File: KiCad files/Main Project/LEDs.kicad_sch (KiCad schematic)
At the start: 11 parts, among them U10 WS2812-4020_dual, U11 WS2812-4020_dual, U12 WS2812-4020_dual, U13 WS2812-4020_dual, U14 WS2812-4020_dual, U15 WS2812-4020_dual, U5 WS2812-4020_dual, U6 WS2812-4020_dual, U7 WS2812-4020_dual, U8 WS2812-4020_dual, U9 WS2812-4020_dual

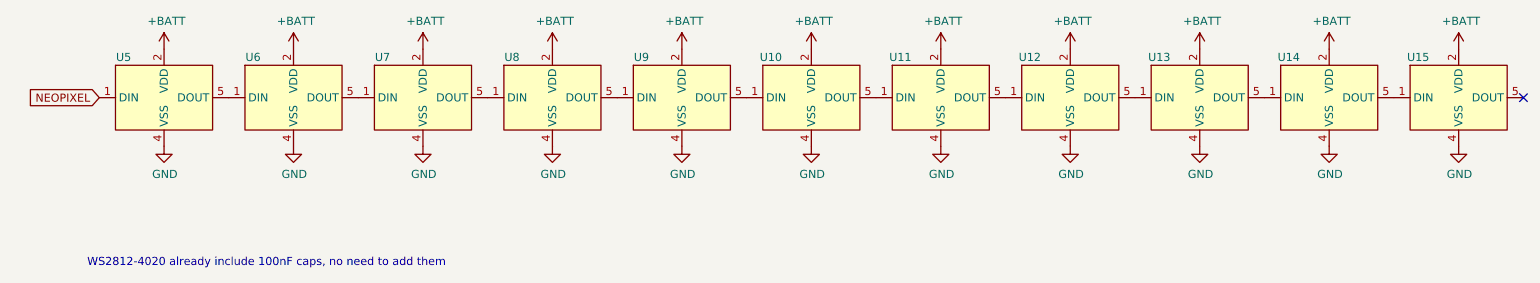
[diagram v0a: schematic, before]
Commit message: update
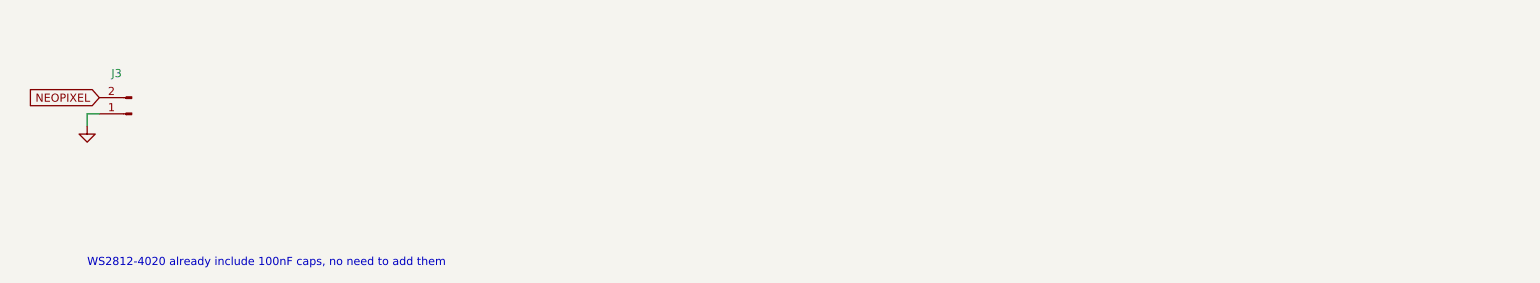
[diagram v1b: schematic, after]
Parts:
- removed U10, U11, U12, U13, U14, U15, U5, U6, U7, U8, U9: WS2812-4020_dual, Josip_global:WS2812-4020-dual-6mm_bezMaske, symbol Josip_symbol_global:WS2812-4020_dual
- added J3: (no value), symbol Connector:Conn_01x02_Male
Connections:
- net GND: now also J3.1 (Pin_1)
- net NEOPIXEL: now also J3.2 (Pin_2)
- no-connect marks 1 -> 0

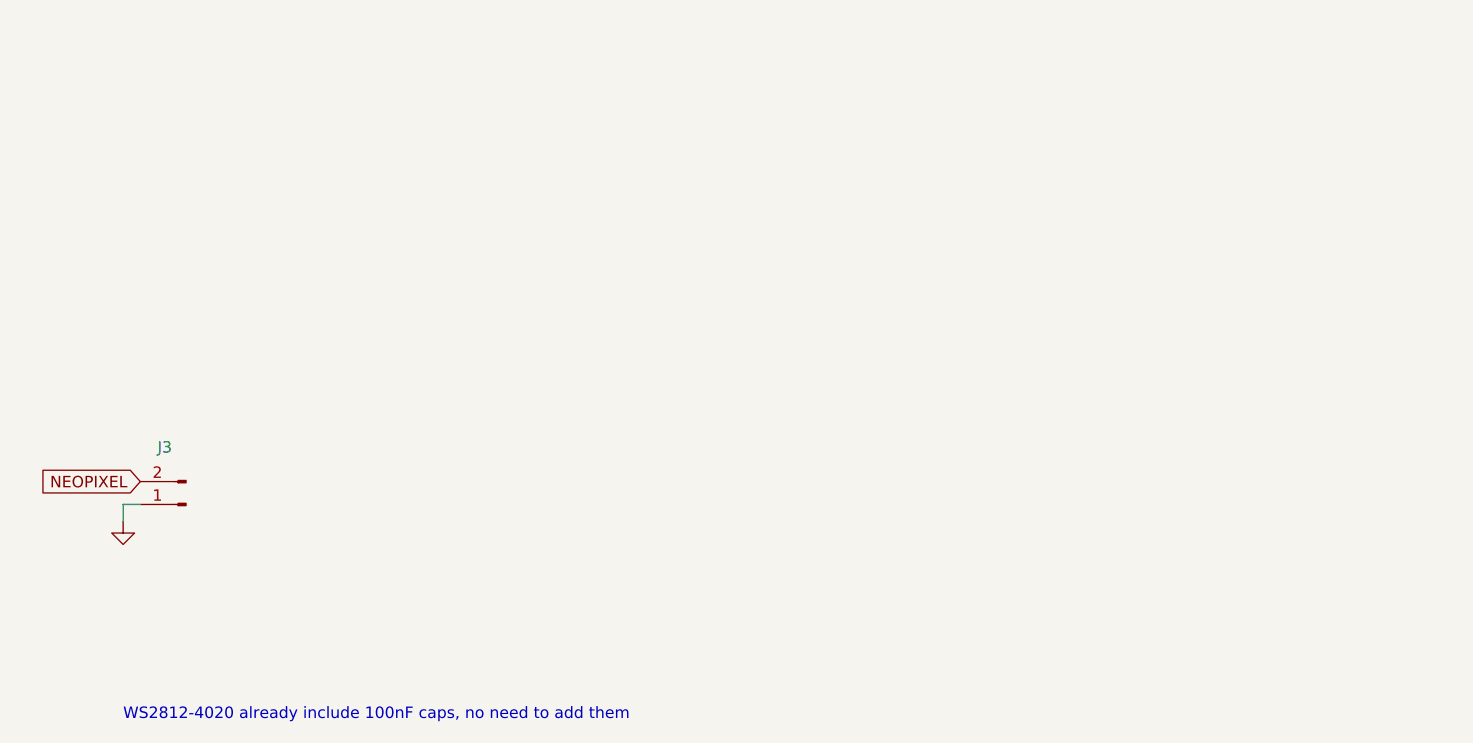
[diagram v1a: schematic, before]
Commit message: update
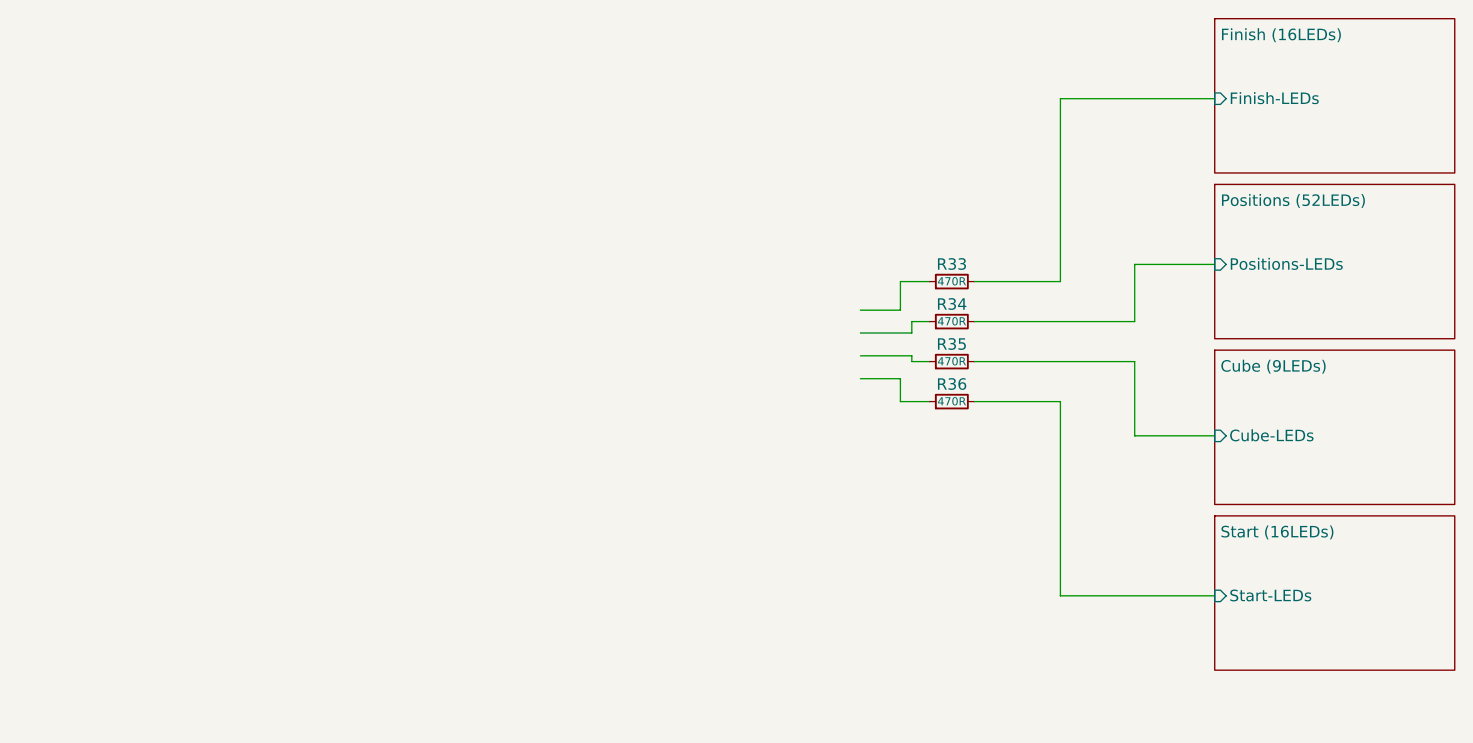
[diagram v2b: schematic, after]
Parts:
- removed J3: (no value), symbol Connector:Conn_01x02_Male
- added R33, R34, R35, R36: 470R, Resistor_SMD:R_0603_1608Metric, symbol Device:R_Small
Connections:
- new net Cube (9LEDs)/Cube-LEDs: R35.2
- new net Finish (16LEDs)/Finish-LEDs: R33.2
- new net Positions (52LEDs)/Positions-LEDs: R34.2
- new net Start (16LEDs)/Start-LEDs: R36.2
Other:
- added sheet Cube (9LEDs) (Cube.kicad_sch)
- added sheet Finish (16LEDs) (Finish.kicad_sch)
- added sheet Positions (52LEDs) (Positions.kicad_sch)
- added sheet Start (16LEDs) (Start.kicad_sch)
- note removed: "WS2812-4020 already include 100nF caps, no need to add them"
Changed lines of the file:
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@@
     (company "Josip&Zvonimir")
   )
-  (wire (pts (xy 42.545 100.965) (xy 42.545 99.06))
+  (wire (pts (xy 146.685 87.63) (xy 137.16 87.63))
     (stroke (width 0) (type default) (color 0 0 0 0))
   )
-  (wire (pts (xy 42.545 99.06) (xy 44.45 99.06))
+  (wire (pts (xy 130.175 80.01) (xy 130.175 78.74))
     (stroke (width 0) (type default) (color 0 0 0 0))
   )
-  (text "WS2812-4020 already include 100nF caps, no need to add them"
-    (at 42.545 123.19 0)
-    (effects (font (size 1.27 1.27)) (justify left bottom))
+  (wire (pts (xy 132.08 87.63) (xy 128.905 87.63))
+    (stroke (width 0) (type default) (color 0 0 0 0))
   )
-  (global_label "NEOPIXEL" (shape input) (at 44.45 96.52 180) (fields_autoplaced)
-    (effects (font (size 1.27 1.27)) (justify right))
-    (property "Intersheet References" "${INTERSHEET_REFS}" (id 0) (at -2.54 50.165 0)
+  (wire (pts (xy 128.905 87.63) (xy 128.905 85.09))
+    (stroke (width 0) (type default) (color 0 0 0 0))
+  )
+  (wire (pts (xy 163.83 72.39) (xy 154.94 72.39))
+    (stroke (width 0) (type default) (color 0 0 0 0))
+  )
+  (wire (pts (xy 137.16 74.295) (xy 146.685 74.295))
+    (stroke (width 0) (type default) (color 0 0 0 0))
+  )
+  (wire (pts (xy 146.685 53.975) (xy 163.83 53.975))
+    (stroke (width 0) (type default) (color 0 0 0 0))
+  )
+  (wire (pts (xy 137.16 83.185) (xy 154.94 83.185))
+    (stroke (width 0) (type default) (color 0 0 0 0))
+  )
+  (wire (pts (xy 124.46 77.47) (xy 128.905 77.47))
+    (stroke (width 0) (type default) (color 0 0 0 0))
+  )
+  (wire (pts (xy 146.685 74.295) (xy 146.685 53.975))
+    (stroke (width 0) (type default) (color 0 0 0 0))
+  )
+  (wire (pts (xy 146.685 109.22) (xy 146.685 87.63))
+    (stroke (width 0) (type default) (color 0 0 0 0))
+  )
+  (wire (pts (xy 128.905 77.47) (xy 128.905 74.295))
+    (stroke (width 0) (type default) (color 0 0 0 0))
+  )
+  (wire (pts (xy 163.83 109.22) (xy 146.685 109.22))
+    (stroke (width 0) (type default) (color 0 0 0 0))
+  )
+  (wire (pts (xy 124.46 82.55) (xy 130.175 82.55))
+    (stroke (width 0) (type default) (color 0 0 0 0))
+  )
+  (wire (pts (xy 124.46 80.01) (xy 130.175 80.01))
+    (stroke (width 0) (type default) (color 0 0 0 0))
+  )
+  (wire (pts (xy 128.905 74.295) (xy 132.08 74.295))
+    (stroke (width 0) (type default) (color 0 0 0 0))
+  )
+  (wire (pts (xy 154.94 83.185) (xy 154.94 91.44))
+    (stroke (width 0) (type default) (color 0 0 0 0))
+  )
+  (wire (pts (xy 154.94 78.74) (xy 137.16 78.74))
+    (stroke (width 0) (type default) (color 0 0 0 0))
+  )
+  (wire (pts (xy 154.94 72.39) (xy 154.94 78.74))
+    (stroke (width 0) (type default) (color 0 0 0 0))
+  )
+  (wire (pts (xy 130.175 78.74) (xy 132.08 78.74))
+    (stroke (width 0) (type default) (color 0 0 0 0))
+  )
+  (wire (pts (xy 154.94 91.44) (xy 163.83 91.44))
+    (stroke (width 0) (type default) (color 0 0 0 0))
+  )
+  (wire (pts (xy 130.175 82.55) (xy 130.175 83.185))
+    (stroke (width 0) (type default) (color 0 0 0 0))
+  )
+  (wire (pts (xy 130.175 83.185) (xy 132.08 83.185))
+    (stroke (width 0) (type default) (color 0 0 0 0))
+  )
+  (wire (pts (xy 128.905 85.09) (xy 124.46 85.09))
+    (stroke (width 0) (type default) (color 0 0 0 0))
+  )
+  (symbol (lib_id "Device:R_Small") (at 134.62 78.74 90) (unit 1)
+    (in_bom yes) (on_board yes)
+    (property "Reference" "R34" (id 0) (at 134.62 76.835 90))
+    (property "Value" "470R" (id 1) (at 134.62 78.74 90)
+      (effects (font (size 0.9 0.9)))
+    )
+    (property "Footprint" "Resistor_SMD:R_0603_1608Metric" (id 2) (at 134.62 78.74 0)
       (effects (font (size 1.27 1.27)) hide)
     )
-  )
-  (symbol (lib_id "Connector:Conn_01x02_Male") (at 49.53 99.06 180) (unit 1)
-    (in_bom yes) (on_board yes)
-    (property "Reference" "J3" (id 0) (at 46.355 92.71 0)
-      (effects (font (size 1.27 1.27)) (justify right))
-    )
-    (property "Value" "" (id 1) (at 50.2412 99.4922 0)
-      (effects (font (size 1.27 1.27)) (justify right) hide)
-    )
-    (property "Footprint" "" (id 2) (at 49.53 99.06 0)
-      (effects (font (size 1.27 1.27)) hide)
-    )
-    (property "Datasheet" "~" (id 3) (at 49.53 99.06 0)
+    (property "Datasheet" "~" (id 3) (at 134.62 78.74 0)
       (effects (font (size 1.27 1.27)) hide)
     )
@@
     (pin "2")
   )
-  (symbol (lib_id "power:GND") (at 42.545 100.965 0) (unit 1)
-    (in_bom yes) (on_board yes) (fields_autoplaced)
-    (property "Reference" "#PWR04" (id 0) (at 42.545 107.315 0)
+  (symbol (lib_id "Device:R_Small") (at 134.62 87.63 90) (unit 1)
+    (in_bom yes) (on_board yes)
+    (property "Reference" "R36" (id 0) (at 134.62 85.725 90))
+    (property "Value" "470R" (id 1) (at 134.62 87.63 90)
+      (effects (font (size 0.9 0.9)))
+    )
+    (property "Footprint" "Resistor_SMD:R_0603_1608Metric" (id 2) (at 134.62 87.63 0)
       (effects (font (size 1.27 1.27)) hide)
     )
-    (property "Value" "" (id 1) (at 42.545 105.4084 0))
-    (property "Footprint" "" (id 2) (at 42.545 100.965 0)
-      (effects (font (size 1.27 1.27)) hide)
-    )
-    (property "Datasheet" "" (id 3) (at 42.545 100.965 0)
+    (property "Datasheet" "~" (id 3) (at 134.62 87.63 0)
       (effects (font (size 1.27 1.27)) hide)
     )
     (pin "1")
+    (pin "2")
+  )
+  (symbol (lib_id "Device:R_Small") (at 134.62 74.295 90) (unit 1)
+    (in_bom yes) (on_board yes)
+    (property "Reference" "R33" (id 0) (at 134.62 72.39 90))
+    (property "Value" "470R" (id 1) (at 134.62 74.295 90)
+      (effects (font (size 0.9 0.9)))
+    )
+    (property "Footprint" "Resistor_SMD:R_0603_1608Metric" (id 2) (at 134.62 74.295 0)
+      (effects (font (size 1.27 1.27)) hide)
+    )
+    (property "Datasheet" "~" (id 3) (at 134.62 74.295 0)
+      (effects (font (size 1.27 1.27)) hide)
+    )
+    (pin "1")
+    (pin "2")
+  )
+  (symbol (lib_id "Device:R_Small") (at 134.62 83.185 90) (unit 1)
+    (in_bom yes) (on_board yes)
+    (property "Reference" "R35" (id 0) (at 134.62 81.28 90))
+    (property "Value" "470R" (id 1) (at 134.62 83.185 90)
+      (effects (font (size 0.9 0.9)))
+    )
+    (property "Footprint" "Resistor_SMD:R_0603_1608Metric" (id 2) (at 134.62 83.185 0)
+      (effects (font (size 1.27 1.27)) hide)
+    )
+    (property "Datasheet" "~" (id 3) (at 134.62 83.185 0)
+      (effects (font (size 1.27 1.27)) hide)
+    )
+    (pin "1")
+    (pin "2")
+  )
+  (sheet (at 163.83 45.085) (size 26.67 17.145)
+    (stroke (width 0.1524) (type solid) (color 0 0 0 0))
+    (fill (color 0 0 0 0.0000))
+    (property "Sheet name" "Finish (16LEDs)" (id 0) (at 164.465 47.625 0)
+      (effects (font (size 1.27 1.27)) (justify left bottom))
+    )
+    (property "Sheet file" "Finish.kicad_sch" (id 1) (at 164.465 59.69 0)
+      (effects (font (size 1.27 1.27)) (justify left top) hide)
+    )
+    (pin "Finish-LEDs" input (at 163.83 53.975 180)
+      (effects (font (size 1.27 1.27)) (justify left))
+    )
+  )
+  (sheet (at 163.83 63.5) (size 26.67 17.145)
+    (stroke (width 0.1524) (type solid) (color 0 0 0 0))
+    (fill (color 0 0 0 0.0000))
+    (property "Sheet name" "Positions (52LEDs)" (id 0) (at 164.465 66.04 0)
+      (effects (font (size 1.27 1.27)) (justify left bottom))
+    )
+    (property "Sheet file" "Positions.kicad_sch" (id 1) (at 164.465 74.93 0)
+      (effects (font (size 1.27 1.27)) (justify left top) hide)
+    )
+    (pin "Positions-LEDs" input (at 163.83 72.39 180)
+      (effects (font (size 1.27 1.27)) (justify left))
+    )
+  )
+  (sheet (at 163.83 100.33) (size 26.67 17.145)
+    (stroke (width 0.1524) (type solid) (color 0 0 0 0))
+    (fill (color 0 0 0 0.0000))
+    (property "Sheet name" "Start (16LEDs)" (id 0) (at 164.465 102.87 0)
+      (effects (font (size 1.27 1.27)) (justify left bottom))
+    )
+    (property "Sheet file" "Start.kicad_sch" (id 1) (at 164.465 114.935 0)
+      (effects (font (size 1.27 1.27)) (justify left top) hide)
+    )
+    (pin "Start-LEDs" input (at 163.83 109.22 180)
+      (effects (font (size 1.27 1.27)) (justify left))
+    )
+  )
+  (sheet (at 163.83 81.915) (size 26.67 17.145)
+    (stroke (width 0.1524) (type solid) (color 0 0 0 0))
+    (fill (color 0 0 0 0.0000))
+    (property "Sheet name" "Cube (9LEDs)" (id 0) (at 164.465 84.455 0)
+      (effects (font (size 1.27 1.27)) (justify left bottom))
+    )
+    (property "Sheet file" "Cube.kicad_sch" (id 1) (at 164.465 93.345 0)
+      (effects (font (size 1.27 1.27)) (justify left top) hide)
+    )
+    (pin "Cube-LEDs" input (at 163.83 91.44 180)
+      (effects (font (size 1.27 1.27)) (justify left))
+    )
   )
 )
